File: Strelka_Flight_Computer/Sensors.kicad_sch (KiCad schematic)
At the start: 8 parts

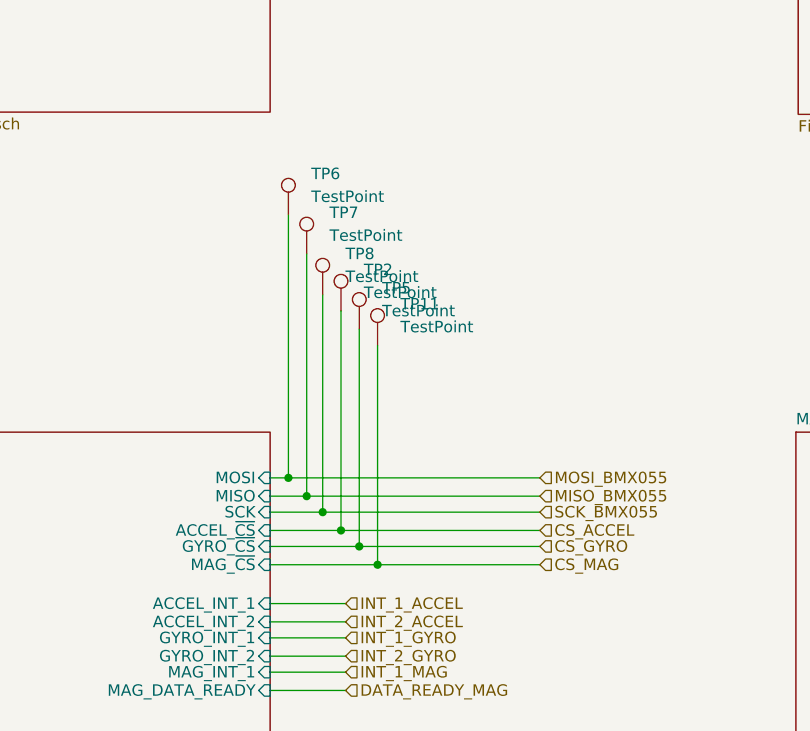
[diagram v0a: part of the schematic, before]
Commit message: Via stitched
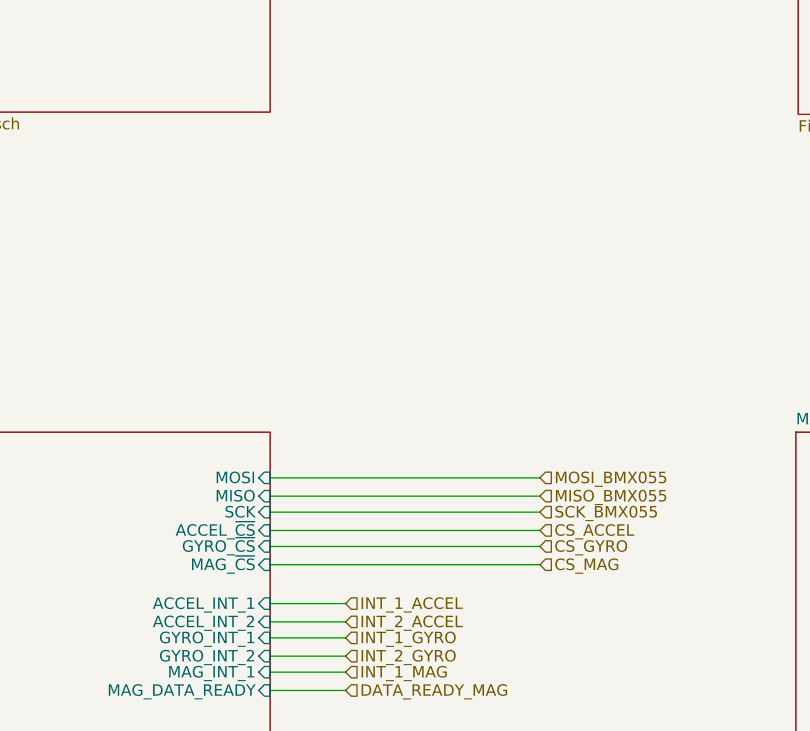
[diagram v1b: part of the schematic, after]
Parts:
- removed TP11, TP2, TP5, TP6, TP7, TP8: TestPoint, TestPoint:TestPoint_Pad_1.0x1.0mm, symbol Connector:TestPoint
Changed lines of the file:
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@@
 (kicad_sch (version 20230121) (generator eeschema)
   (paper "A4")
-  (junction (at 107.188 122.682) (diameter 0) (color 0 0 0 0)
-  )
-  (junction (at 103.124 118.872) (diameter 0) (color 0 0 0 0)
-  )
   (junction (at 217.932 120.142) (diameter 0) (color 0 0 0 0)
   )
-  (junction (at 105.156 120.65) (diameter 0) (color 0 0 0 0)
-  )
-  (junction (at 101.092 116.84) (diameter 0) (color 0 0 0 0)
-  )
   (junction (at 212.852 121.92) (diameter 0) (color 0 0 0 0)
   )
-  (junction (at 97.282 113.03) (diameter 0) (color 0 0 0 0)
-  )
-  (junction (at 99.314 115.062) (diameter 0) (color 0 0 0 0)
-  )
   (no_connect (at 211.582 125.73))
-  (wire (pts (xy 107.188 98.298) (xy 107.188 122.682))
-    (stroke (width 0) (type default))
-  )
-  (wire (pts (xy 95.25 115.062) (xy 99.314 115.062))
-    (stroke (width 0) (type default))
-  )
-  (wire (pts (xy 105.156 120.65) (xy 125.222 120.65))
+  (wire (pts (xy 95.25 115.062) (xy 125.222 115.062))
     (stroke (width 0) (type default))
   )
@@
     (stroke (width 0) (type default))
   )
-  (wire (pts (xy 95.25 116.84) (xy 101.092 116.84))
+  (wire (pts (xy 95.25 116.84) (xy 125.222 116.84))
     (stroke (width 0) (type default))
   )
@@
     (stroke (width 0) (type default))
   )
-  (wire (pts (xy 105.156 96.52) (xy 105.156 120.65))
-    (stroke (width 0) (type default))
-  )
   (wire (pts (xy 217.932 113.792) (xy 217.932 120.142))
     (stroke (width 0) (type default))
   )
-  (wire (pts (xy 103.124 94.488) (xy 103.124 118.872))
-    (stroke (width 0) (type default))
-  )
-  (wire (pts (xy 97.282 83.82) (xy 97.282 113.03))
-    (stroke (width 0) (type default))
-  )
   (wire (pts (xy 95.25 45.212) (xy 103.632 45.212))
     (stroke (width 0) (type default))
@@
     (stroke (width 0) (type default))
   )
-  (wire (pts (xy 99.314 115.062) (xy 125.222 115.062))
-    (stroke (width 0) (type default))
-  )
-  (wire (pts (xy 107.188 122.682) (xy 125.222 122.682))
-    (stroke (width 0) (type default))
-  )
-  (wire (pts (xy 95.25 113.03) (xy 97.282 113.03))
-    (stroke (width 0) (type default))
-  )
-  (wire (pts (xy 97.282 113.03) (xy 125.222 113.03))
+  (wire (pts (xy 95.25 113.03) (xy 125.222 113.03))
     (stroke (width 0) (type default))
   )
@@
     (stroke (width 0) (type default))
   )
-  (wire (pts (xy 101.092 116.84) (xy 125.222 116.84))
-    (stroke (width 0) (type default))
-  )
   (wire (pts (xy 211.582 120.142) (xy 217.932 120.142))
     (stroke (width 0) (type default))
@@
     (stroke (width 0) (type default))
   )
-  (wire (pts (xy 99.314 88.138) (xy 99.314 115.062))
-    (stroke (width 0) (type default))
-  )
   (wire (pts (xy 211.582 48.641) (xy 219.964 48.641))
     (stroke (width 0) (type default))
@@
     (stroke (width 0) (type default))
   )
-  (wire (pts (xy 95.25 120.65) (xy 105.156 120.65))
-    (stroke (width 0) (type default))
-  )
-  (wire (pts (xy 95.25 122.682) (xy 107.188 122.682))
-    (stroke (width 0) (type default))
-  )
-  (wire (pts (xy 95.25 118.872) (xy 103.124 118.872))
+  (wire (pts (xy 95.25 120.65) (xy 125.222 120.65))
+    (stroke (width 0) (type default))
+  )
+  (wire (pts (xy 95.25 122.682) (xy 125.222 122.682))
+    (stroke (width 0) (type default))
+  )
+  (wire (pts (xy 95.25 118.872) (xy 125.222 118.872))
     (stroke (width 0) (type default))
   )
@@
   )
   (wire (pts (xy 211.582 118.11) (xy 219.71 118.11))
-    (stroke (width 0) (type default))
-  )
-  (wire (pts (xy 103.124 118.872) (xy 125.222 118.872))
-    (stroke (width 0) (type default))
-  )
-  (wire (pts (xy 101.092 92.71) (xy 101.092 116.84))
     (stroke (width 0) (type default))
   )
@@
         )
       )
-    )
-  )
-  (symbol (lib_id "Connector:TestPoint") (at 101.092 92.71 0) (unit 1)
-    (in_bom yes) (on_board yes) (dnp no) (fields_autoplaced)
-    (property "Reference" "TP8" (at 103.632 88.1379 0)
-      (effects (font (size 1.27 1.27)) (justify left))
-    )
-    (property "Value" "TestPoint" (at 103.632 90.6779 0)
-      (effects (font (size 1.27 1.27)) (justify left))
-    )
-    (property "Footprint" "TestPoint:TestPoint_Pad_1.0x1.0mm" (at 106.172 92.71 0)
-      (effects (font (size 1.27 1.27)) hide)
-    )
-    (property "Datasheet" "~" (at 106.172 92.71 0)
-      (effects (font (size 1.27 1.27)) hide)
-    )
-    (pin "1")
-    (instances
-      (project "Strelka_Flight_Computer"
-        (path "/e63e39d7-6ac0-4ffd-8aa3-1841a4541b55/78f71895-bddb-4f64-a608-99074f2d1c44"
-          (reference "TP8") (unit 1)
-        )
-      )
-    )
-  )
-  (symbol (lib_id "Connector:TestPoint") (at 107.188 98.298 0) (unit 1)
-    (in_bom yes) (on_board yes) (dnp no) (fields_autoplaced)
-    (property "Reference" "TP11" (at 109.728 93.7259 0)
-      (effects (font (size 1.27 1.27)) (justify left))
-    )
-    (property "Value" "TestPoint" (at 109.728 96.2659 0)
-      (effects (font (size 1.27 1.27)) (justify left))
-    )
-    (property "Footprint" "TestPoint:TestPoint_Pad_1.0x1.0mm" (at 112.268 98.298 0)
-      (effects (font (size 1.27 1.27)) hide)
-    )
-    (property "Datasheet" "~" (at 112.268 98.298 0)
-      (effects (font (size 1.27 1.27)) hide)
-    )
-    (pin "1")
-    (instances
-      (project "Strelka_Flight_Computer"
-        (path "/e63e39d7-6ac0-4ffd-8aa3-1841a4541b55/78f71895-bddb-4f64-a608-99074f2d1c44"
-          (reference "TP11") (unit 1)
-        )
-      )
-    )
-  )
-  (symbol (lib_id "Connector:TestPoint") (at 105.156 96.52 0) (unit 1)
-    (in_bom yes) (on_board yes) (dnp no) (fields_autoplaced)
-    (property "Reference" "TP5" (at 107.696 91.9479 0)
-      (effects (font (size 1.27 1.27)) (justify left))
-    )
-    (property "Value" "TestPoint" (at 107.696 94.4879 0)
-      (effects (font (size 1.27 1.27)) (justify left))
-    )
-    (property "Footprint" "TestPoint:TestPoint_Pad_1.0x1.0mm" (at 110.236 96.52 0)
-      (effects (font (size 1.27 1.27)) hide)
-    )
-    (property "Datasheet" "~" (at 110.236 96.52 0)
-      (effects (font (size 1.27 1.27)) hide)
-    )
-    (pin "1")
-    (instances
-      (project "Strelka_Flight_Computer"
-        (path "/e63e39d7-6ac0-4ffd-8aa3-1841a4541b55/78f71895-bddb-4f64-a608-99074f2d1c44"
-          (reference "TP5") (unit 1)
-        )
-      )
-    )
-  )
-  (symbol (lib_id "Connector:TestPoint") (at 99.314 88.138 0) (unit 1)
-    (in_bom yes) (on_board yes) (dnp no) (fields_autoplaced)
-    (property "Reference" "TP7" (at 101.854 83.5659 0)
-      (effects (font (size 1.27 1.27)) (justify left))
-    )
-    (property "Value" "TestPoint" (at 101.854 86.1059 0)
-      (effects (font (size 1.27 1.27)) (justify left))
-    )
-    (property "Footprint" "TestPoint:TestPoint_Pad_1.0x1.0mm" (at 104.394 88.138 0)
-      (effects (font (size 1.27 1.27)) hide)
-    )
-    (property "Datasheet" "~" (at 104.394 88.138 0)
-      (effects (font (size 1.27 1.27)) hide)
-    )
-    (pin "1")
-    (instances
-      (project "Strelka_Flight_Computer"
-        (path "/e63e39d7-6ac0-4ffd-8aa3-1841a4541b55/78f71895-bddb-4f64-a608-99074f2d1c44"
-          (reference "TP7") (unit 1)
-        )
-      )
-    )
-  )
-  (symbol (lib_id "Connector:TestPoint") (at 103.124 94.488 0) (unit 1)
-    (in_bom yes) (on_board yes) (dnp no) (fields_autoplaced)
-    (property "Reference" "TP2" (at 105.664 89.9159 0)
-      (effects (font (size 1.27 1.27)) (justify left))
-    )
-    (property "Value" "TestPoint" (at 105.664 92.4559 0)
-      (effects (font (size 1.27 1.27)) (justify left))
-    )
-    (property "Footprint" "TestPoint:TestPoint_Pad_1.0x1.0mm" (at 108.204 94.488 0)
-      (effects (font (size 1.27 1.27)) hide)
-    )
-    (property "Datasheet" "~" (at 108.204 94.488 0)
-      (effects (font (size 1.27 1.27)) hide)
-    )
-    (pin "1")
-    (instances
-      (project "Strelka_Flight_Computer"
-        (path "/e63e39d7-6ac0-4ffd-8aa3-1841a4541b55/78f71895-bddb-4f64-a608-99074f2d1c44"
-          (reference "TP2") (unit 1)
-        )
-      )
-    )
-  )
-  (symbol (lib_id "Connector:TestPoint") (at 97.282 83.82 0) (unit 1)
-    (in_bom yes) (on_board yes) (dnp no) (fields_autoplaced)
-    (property "Reference" "TP6" (at 99.822 79.2479 0)
-      (effects (font (size 1.27 1.27)) (justify left))
-    )
-    (property "Value" "TestPoint" (at 99.822 81.7879 0)
-      (effects (font (size 1.27 1.27)) (justify left))
-    )
-    (property "Footprint" "TestPoint:TestPoint_Pad_1.0x1.0mm" (at 102.362 83.82 0)
-      (effects (font (size 1.27 1.27)) hide)
-    )
-    (property "Datasheet" "~" (at 102.362 83.82 0)
-      (effects (font (size 1.27 1.27)) hide)
-    )
-    (pin "1")
-    (instances
-      (project "Strelka_Flight_Computer"
-        (path "/e63e39d7-6ac0-4ffd-8aa3-1841a4541b55/78f71895-bddb-4f64-a608-99074f2d1c44"
-          (reference "TP6") (unit 1)
-        )
-      )
